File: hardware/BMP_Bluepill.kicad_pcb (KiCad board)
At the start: 2 copper layers, 42.3 x 20 mm, 30 parts, among them J1 Conn_01x06, J2 USB_C_Receptacle_USB2.0_16P, J3 Conn_01x04, U1 STM32F103C8T6, U2 AMS1117-3.3, Y1 8 MHz

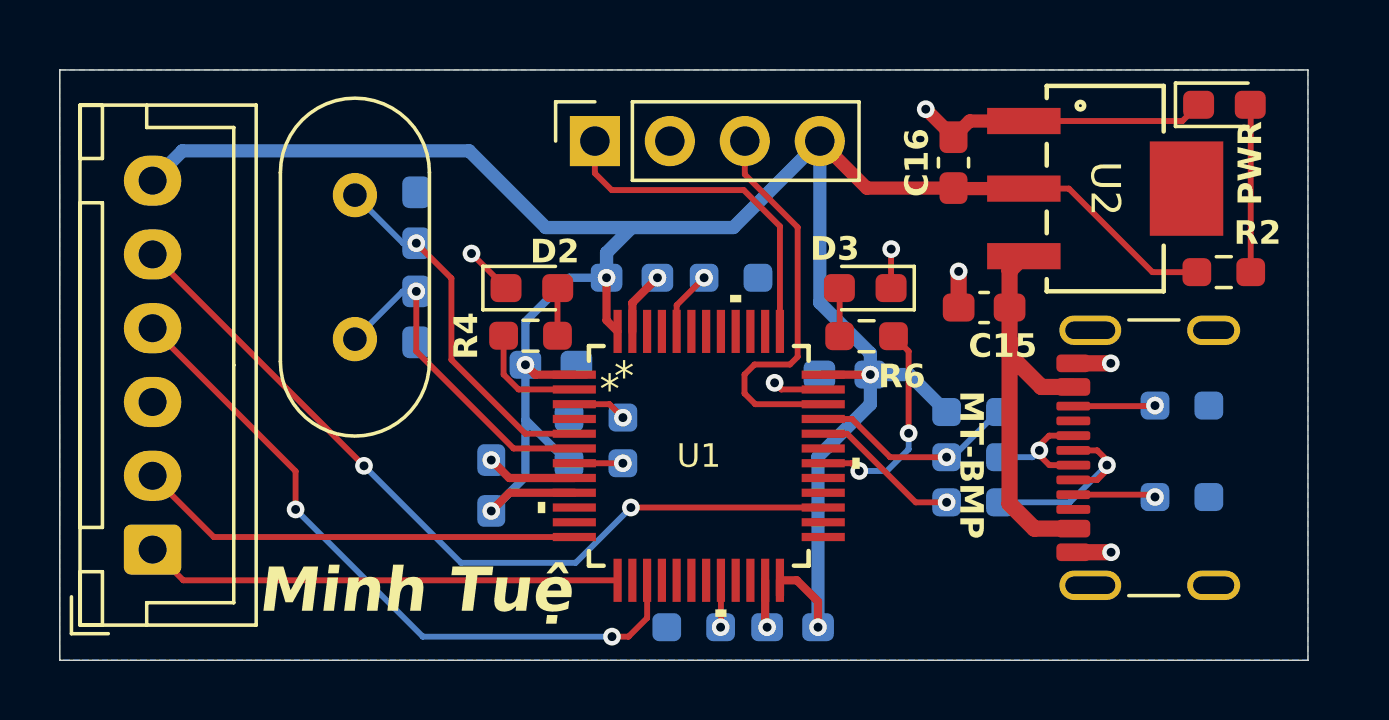
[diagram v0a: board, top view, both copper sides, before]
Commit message: update layout
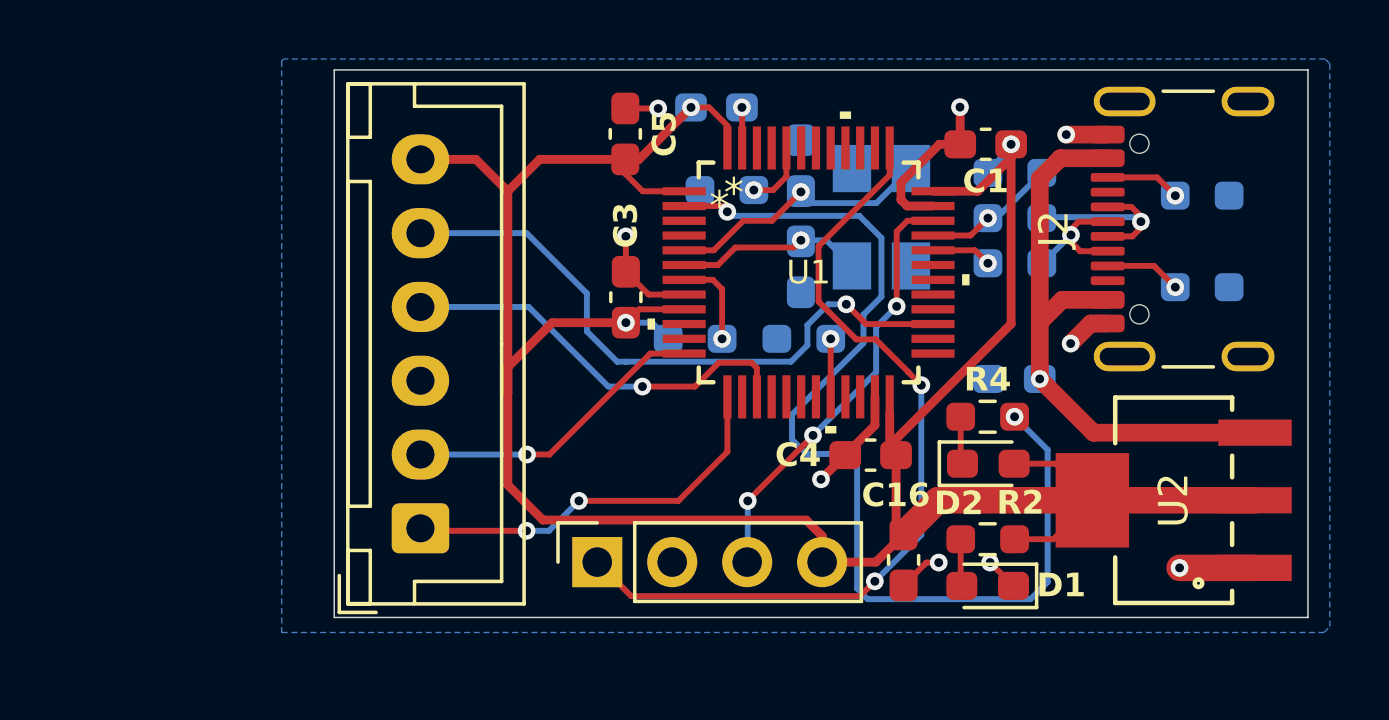
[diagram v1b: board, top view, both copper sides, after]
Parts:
- removed D3: LED, LED_SMD:LED_0603_1608Metric_Pad1.05x0.95mm_HandSolder
- removed R5: 10k[N/A], Resistor_SMD:R_0603_1608Metric_Pad0.98x0.95mm_HandSolder
- removed R6: 1k, Resistor_SMD:R_0603_1608Metric_Pad0.98x0.95mm_HandSolder
- removed Y1: 8 MHz, Crystal:Crystal_HC49-4H_Vertical
- added Y2: 8MHz, Crystal:Crystal_SMD_5032-4Pin_5.0x3.2mm, B.Cu at (127.8, 105.0)
- C1, C3, C4, C5: moved to F.Cu
- C15: moved to B.Cu
- moved D1 18.2 mm to (131.4, 117.5), turned to 180 degrees
- moved D2 16.6 mm to (131.5, 113.3)
- moved R4 15.7 mm to (131.4, 111.8), turned to 180 degrees
- moved J3 14.3 mm to (118.2, 116.7)
- moved C16 13.6 mm to (128.6, 116.6), turned to -90 degrees
- moved C13 13.1 mm to (125.1, 103.2)
- moved C14 13.1 mm to (125.1, 106.7)
- moved C5 12.7 mm to (119.2, 102.2)
- moved R2 12.1 mm to (131.4, 115.9), turned to 180 degrees
- moved U2 10.8 mm to (137.7, 114.6), turned to 90 degrees
- moved R7 10.5 mm to (125.2, 109.1)
- moved C2 10.4 mm to (122.2, 101.3)
- moved C1 9.14 mm to (131.4, 102.5)
- moved J1 9.10 mm to (112.2, 115.5)
- moved R16 8.22 mm to (132.4, 105.0)
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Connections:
- D2 pad 1: GND -> Net-(D2-K)
- D2 pad 2: Net-(D2-A) -> +3V3
- J2 pad S1: unconnected-(J2-SHIELD-PadS1)_3 -> GND
- R4 pad 2: Net-(D2-A) -> Net-(D2-K)
- U1 pad 3: Net-(U1A-PC14-OSC32_IN) -> unconnected-(U1A-PC14-OSC32_IN-Pad3)
- U1 pad 30: LED_UART -> unconnected-(U1A-PA9-Pad30)
- U2 pad 4: unconnected-(U2-EPAD-Pad4) -> +3V3
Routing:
- net LED_IDLE: track 3.92 -> 34.8 mm, vias 0 -> 2
- net SWD_CLK: track 11.7 -> 28.2 mm, vias 0 -> 2
- net BMP_CLK: track 23.4 -> 13.9 mm, vias 2 -> 1
- net LED_UART: track 7.35 -> 0.00 mm, vias 2 -> 0
- net BMP_IO: track 27.8 -> 21.4 mm, vias 2 -> 1
- net +5V: track 14.2 -> 20.0 mm, vias 0 -> 1
- net Net-(U1A-OSC_OUT): track 11.5 -> 6.42 mm
- net BMP_TX: track 15.1 -> 10.4 mm, vias 0 -> 1
- net Net-(D1-A): track 5.68 -> 1.60 mm
- net +3V3: track 86.8 -> 90.5 mm, vias 5 -> 3
- net Net-(U1A-OSC_IN): track 12.4 -> 9.13 mm
- net USB-: track 5.14 -> 2.04 mm
- net BMP_RX: track 16.2 -> 13.4 mm, vias 0 -> 2
- net USB+: track 7.18 -> 4.56 mm
- net Net-(J2-D--PadA7): track 7.02 -> 4.68 mm
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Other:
- board size 42.3 x 20 mm -> 33 x 18.5 mm
- board text removed: "MT-BMP"
- board text removed: "PWR"
